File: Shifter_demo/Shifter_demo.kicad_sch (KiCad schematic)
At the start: 37 parts, among them IC1 BD450M2WFP3-CE2, IC2 LMR50410Y3FQDBVRQ1, J1 GT-USB-7010AN, SW1 TL3302BF180QG, SW2 TL3302BF180QG, U1 RP2040, U3 W25Q128JVSIQ, X1 XTAL12MHZ

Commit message: Add files via upload
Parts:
- added D1: RED LED, LED_SMD:LED_0805_2012Metric_Pad1.15x1.40mm_HandSolder, symbol Device:LED
- added D2: GREEN LED, LED_SMD:LED_0805_2012Metric_Pad1.15x1.40mm_HandSolder, symbol Device:LED
- added D3: BLUE LED, LED_SMD:LED_0805_2012Metric_Pad1.15x1.40mm_HandSolder, symbol Device:LED
- added J2, J3: B03B-XASK-1_LF__SN_, Connector_JST:JST_XA_B03B-XASK-1_1x03_P2.50mm_Vertical, symbol B03B-XASK-1_LF__SN_:B03B-XASK-1_LF__SN_
- added R10: 270R, Resistor_SMD:R_0805_2012Metric_Pad1.20x1.40mm_HandSolder, symbol Device:R
- added R11: 220R, Resistor_SMD:R_0805_2012Metric_Pad1.20x1.40mm_HandSolder, symbol Device:R
- added R13: 100R, Resistor_SMD:R_0805_2012Metric_Pad1.20x1.40mm_HandSolder, symbol Device:R
- added S1, S2: KMR731NG_LFS, KMR731NG LFS:KMR731NGLFS, symbol KMR731NG_LFS:KMR731NG_LFS
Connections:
- net +3V3: now also R10.1
- net GND: now also D1.1 (K), D2.1 (K), D3.1 (K), J2.1, J3.1, S1.1 (NO_1), S1.2 (NO_2), S1.3 (COM_1), S2.1 (NO_1), S2.2 (NO_2), S2.3 (COM_1)
- net Test_UP_Button: now reaches U1.3 (GPIO1)
- net Test_UP_Button: now also S1.4 (COM_2)
- net Test_DOWN_Button: now reaches U1.4 (GPIO2)
- net Test_DOWN_Button: now also S2.4 (COM_2)
- net UP_Button: now reaches U1.5 (GPIO3)
- net DOWN_Button: now reaches U1.6 (GPIO4)
- net DOWN_LED: now reaches U1.8 (GPIO6)
- net DOWN_LED: now also R13.1
- net UP_LED: now reaches U1.9 (GPIO7)
- net UP_LED: now also R11.1
- new net: D1.2 (A), R10.2
- new net: D3.2 (A), R13.2
- new net: D2.2 (A), R11.2
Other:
- note added: "Buttons"
- note added: "ECU wires can be 5-14 V + nasty spikes, so cant connect directly. aka we need to use interface circuitry For analog sensors: high-value voltage divider + RC filter so the RP2040s ADC never sees over 3.3 V and doesn't load the sensor. For buses like CAN/LIN, we need proper transceiver ICs."
- note added: "I went with: POWER: RED(Constant) UP: GREEN(One Blink) DOWN: BLUE(One Blink)"
- note added: "Idk what u want to conect here, but there u are:"
- note added: "JST XAs"
- note added: "LEDs"
- note added: "Original"
- note added: "The buttons are active low"
- moved on the sheet: C1, C10, C11, C12, C13, C14, C15, C16, C17, C18, C2, C3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

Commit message: Update Schematic
Adds ESP32, CAN and basically everything...
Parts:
- removed C1, C9: 1u, C0603, symbol Reference_import-altium-import:root_3_CL10A105KB8NNNC_
- removed C10, C11, C14: 100n, C0603, symbol Reference_import-altium-import:root_1_CC0603KRX7R9BB104_
- removed C12, C13: 27P, C0603, symbol Reference_import-altium-import:root_0_CL10C270JB8NNNC_
- removed C2, C3, C4, C5, C6, C7, C8: 100n, C0603, symbol Reference_import-altium-import:root_3_CC0603KRX7R9BB104_
- removed IC1: BD450M2WFP3-CE2, SOT230P700X170-4N, symbol BD450M2WFP3-CE2:BD450M2WFP3-CE2
- removed J1: GT-USB-7010AN, USB-SMD_GT-USB-7010AN, symbol Reference_import-altium-import:root_0_GT-USB-7010AN_
- removed J2, J3: B03B-XASK-1_LF__SN_, Connector_JST:JST_XA_B03B-XASK-1_1x03_P2.50mm_Vertical, symbol B03B-XASK-1_LF__SN_:B03B-XASK-1_LF__SN_
- removed R1, R2: 27, R0603, symbol Reference_import-altium-import:root_0_0603WAF270JT5E_
- removed R12: 10k, R0603, symbol Reference_import-altium-import:root_1_0603WAF1002T5E_
- removed R3, R5: 1k, R0603, symbol Reference_import-altium-import:root_0_0603WAF1001T5E_
- removed R4: 10k - DNF, R0603, symbol Reference_import-altium-import:root_1_10k - DNF_
- removed S1, S2: KMR731NG_LFS, KMR731NG LFS:KMR731NGLFS, symbol KMR731NG_LFS:KMR731NG_LFS
- removed SW1: TL3302BF180QG, SW-SMD_L6.0-W3.5-LS10.2, symbol Reference_import-altium-import:root_0_TL3302BF180QG_
- removed SW2: TL3302BF180QG, SW-SMD_L6.0-W3.5-LS10.2, symbol Reference_import-altium-import:root_1_TL3302BF180QG_
- removed U1: RP2040, symbol Reference_import-altium-import:root_0_RP2040_
- removed U3: W25Q128JVSIQ, SOIC-8_L5.3-W5.3-P1.27-LS8.0-BL, symbol Reference_import-altium-import:root_0_W25Q128JVSSIQ_
- removed X1: XTAL12MHZ, CRYSTAL-SMD_4P-L2.5-W2.0-BL_XTAL12MHZ, symbol Reference_import-altium-import:root_0_XTAL12MHz_
- added C1, C5: 1u, symbol Device:C
- added C2: 22u, symbol Device:C
- added C3, C4, C6, C7, C8: 0.1u, symbol Device:C
- added D4: RED LED, LED_SMD:LED_0805_2012Metric_Pad1.15x1.40mm_HandSolder, symbol Device:LED
- added J1: RST, symbol Connector_Generic:Conn_01x02
- added J2: BSEL, symbol Connector_Generic:Conn_01x02
- added J3: S06B-XASK-1, symbol Connector_Generic:Conn_01x06
- added J4: SO4B-XASK-1, symbol Connector_Generic:Conn_01x04
- added J5, J6: S03B-XASK-1, symbol Connector_Generic:Conn_01x03
- added Q1: BSS205N, Custom_MSM:MOSFET_Single_SOT-23, symbol Custom_MSM:MOSFET_N-CH
- added R1, R2: 27, symbol Device:R
- added R3: 10k, symbol Device:R
- added R4: 270R, Resistor_SMD:R_0805_2012Metric_Pad1.20x1.40mm_HandSolder, symbol Device:R
- added U1: ESP32-S3-WROOM-1U-N4R2, ESP32-S3-WROOM-1U-N4R2:XCVR_ESP32-S3-WROOM-1U-N4R2, symbol ESP32-S3-WROOM-1U-N4R2:ESP32-S3-WROOM-1U-N4R2
- added U3: MAX3390EEUD_T, MAX3390EEUD_T:SOP65P640X110-14N, symbol MAX3390EEUD_T:MAX3390EEUD_T
- added U4: ISO1042BQDWVQ1, DWV0008A-IPC_A, symbol 2025-11-15_02-18-59:ISO1042BQDWVQ1
- added USB1: GT-USB-7010AN, USB-SMD_GT-USB-7010AN, symbol Reference_import-altium-import:root_0_GT-USB-7010AN_
- renumbered IC2 to U2
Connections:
- net +3V3: now also C2.2, C3.2, C6.1, C8.2, R3.1, U1.2 (3V3), U3.1 (VL), U3.8 (~{THREE}-STATE), U4.1 (VCC1)
- net +5V: now also C4.1, C5.1, C7.2, J3.6 (Pin_6), J5.3 (Pin_3), U3.14 (VCC), U4.8 (VCC2), USB1.A4B9 (VBUS), USB1.B4A9 (VBUS)
- net DOWN_LED: now also U1.7 (IO7)
- net GND: now also C1.1, C2.1, C3.1, C4.2, C5.2, C6.2, C7.1, C8.1, D4.1 (K), J1.1 (Pin_1), J2.1 (Pin_1), J3.1 (Pin_1), J5.1 (Pin_1), J6.1 (Pin_1), Q1.2 (S), U1.1 (GND), U1.40 (GND__1), U1.41_1 (GND__2), U1.41_2 (GND__3), U1.41_3 (GND__4), U1.41_4 (GND__5), U1.41_5 (GND__6), U1.41_6 (GND__7), U1.41_7 (GND__8), U1.41_8 (GND__9), U1.41_9 (GND__10), U3.7 (GND), U4.4 (GND1), U4.5 (GND2), USB1.13 (GND), USB1.14 (GND), USB1.15 (GND), USB1.16 (GND), USB1.A1B12 (GND), USB1.B1A12 (GND)
- net SCLK: now also U1.20 (IO12), U3.4 (I_VL3)
- net UP_LED: now also U1.6 (IO6)
- net USBD+: now also R2.2, USB1.A6 (DP1), USB1.B6 (DP2)
- net USBD-: now also R1.2, USB1.A7 (DN1), USB1.B7 (DN2)
- net at R8.2: now also USB1.A5 (CC1)
- net at R7.2: now also USB1.B5 (CC2)
- new net: R1.1, U1.13 (IO19)
- new net: D4.2 (A), R4.2
- new net: R2.1, U1.14 (IO20)
- new net: J2.2 (Pin_2), U1.27 (IO0)
- new net CAND: U1.39 (IO1), U4.2 (TXD)
- new net CANH: J6.3 (Pin_3), U4.7 (CANH)
- new net CANL: J6.2 (Pin_2), U4.6 (CANL)
- new net CANR: U1.38 (IO2), U4.3 (RXD)
- new net CS: U1.18 (IO10), U3.5 (I_VL4)
- new net ECU: J4.4 (Pin_4), Q1.3 (D)
- new net E_CS: J3.5 (Pin_5), U3.10 (O_VCC4)
- new net E_MISO: J3.3 (Pin_3), U3.13 (I_VCC1)
- new net E_MOSI: J3.4 (Pin_4), U3.12 (O_VCC2)
- new net E_SCLK: J3.2 (Pin_2), U3.11 (O_VCC3)
- new net FLATSHIFT: Q1.1 (G), U1.5 (IO5)
- new net MISO: U1.21 (IO13), U3.2 (O_VL1)
- new net MOSI: U1.19 (IO11), U3.3 (I_VL2)
- new net Main_Reset: C1.2, J1.2 (Pin_2), R3.2, U1.3 (EN)
- new net NEUTRAL: J4.1 (Pin_1)
- new net NEUTRAL_LED: R4.1, U1.12 (IO8)
- new net PWM: J5.2 (Pin_2)
- new net RX: U1.36 (RXD0)
- new net SHIFT_DOWN: J4.2 (Pin_2)
- new net SHIFT_UP: J4.3 (Pin_3)
- new net TX: U1.37 (TXD0)
- no-connect marks 32 -> 23
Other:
- note added: "CAN"
- note added: "CAN (Rest of Car)"
- note added: "ECU"
- note added: "ESC"
- note added: "Encoder"
- note added: "Encoder Interface"
- note added: "Microcontroller"
- note added: "REG"
- note added: "Rest of Car"
- note added: "USB"
- note removed: "Buttons"
- note removed: "C1 must be near Pin 44"
- note removed: "C9 must be near Pin 45"
- note removed: "ECU wires can be 5-14 V + nasty spikes, so cant connect directly. aka we need to use interface circuitry For analog sensors: high-value voltage divider + RC filter so the RP2040s ADC never sees over 3.3 V and doesn't load the sensor. For buses like CAN/LIN, we need proper transceiver ICs."
- note removed: "Idk what u want to conect here, but there u are:"
- note removed: "Linear Batt to 5V reg"
- note removed: "On-PCB shifter buttons (For testing) ECU signal line (research required) Status Lights Connectors (JST XA)"
- note removed: "Original"
- note removed: "R1 and R2 must be near RP2040"
- note removed: "RP2040 Microcontroller"
- note removed: "SPI Flash"
- note removed: "Switching 5V to 3V3 reg"
- note removed: "The buttons are active low"
- note removed: "Todo:"
- note removed: "Try to match crystal track length"
- note removed: "USB BOOT (Pull Low)"
- moved on the sheet: C15, C16, C17, C18, D1, D2, D3, L1, R10, R11, R13, R6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

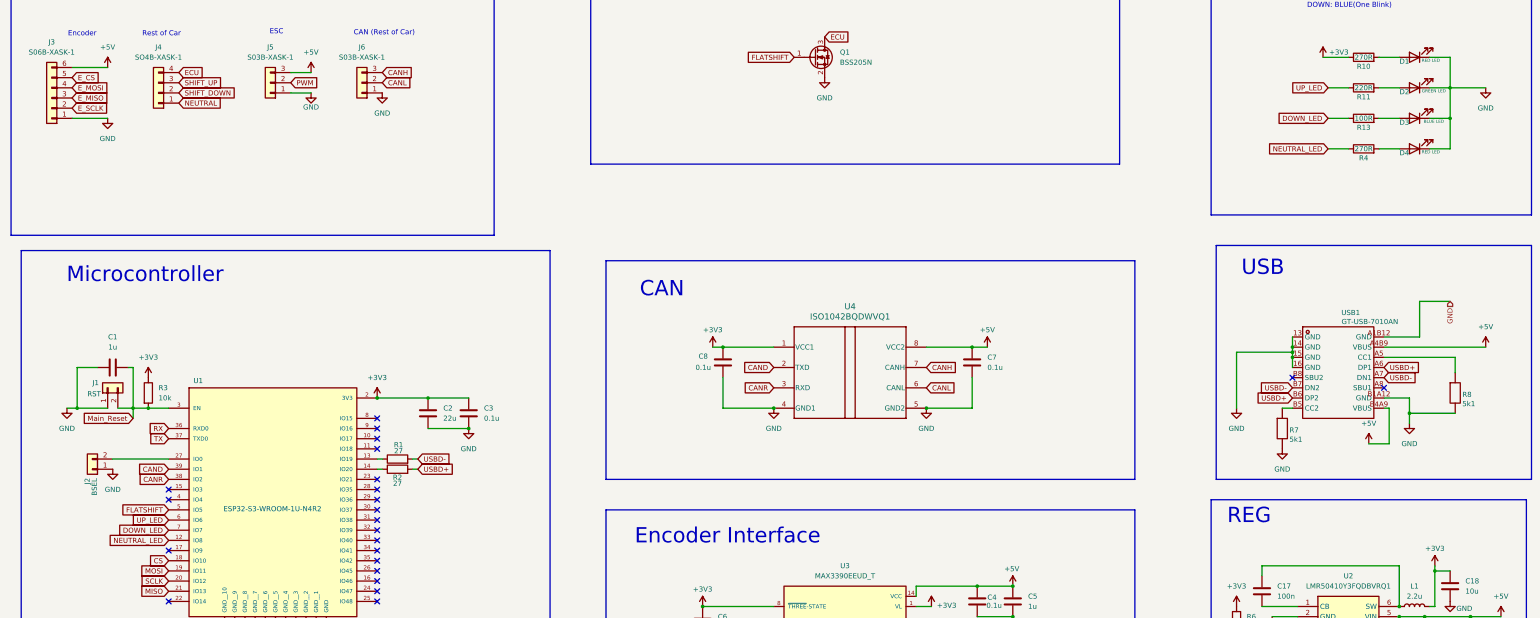
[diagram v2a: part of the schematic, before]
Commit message: route it all and make minor schem mods
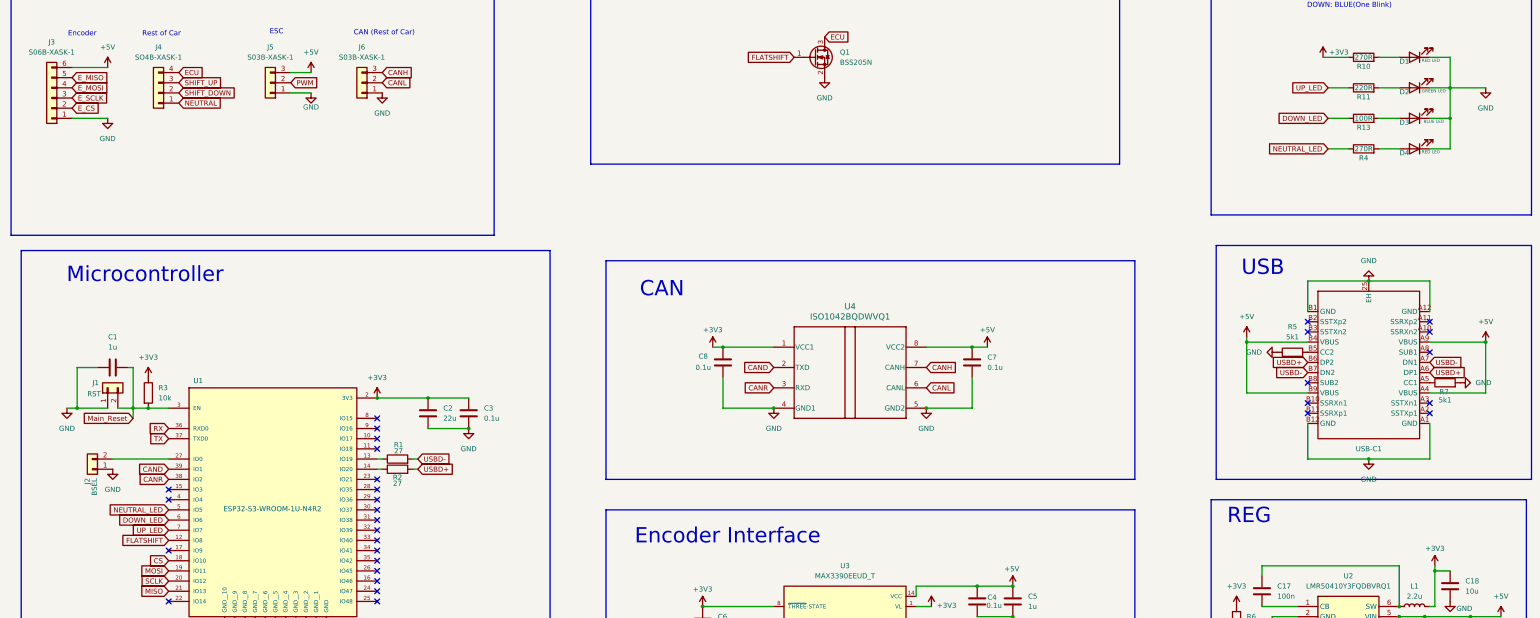
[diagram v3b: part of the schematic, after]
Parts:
- removed R7, R8: 5k1, R0603, symbol Reference_import-altium-import:root_1_0603WAF5101T5E_
- removed USB1: GT-USB-7010AN, USB-SMD_GT-USB-7010AN, symbol Reference_import-altium-import:root_0_GT-USB-7010AN_
- added R5, R7: 5k1, Resistor_SMD:R_0805_2012Metric_Pad1.20x1.40mm_HandSolder, symbol Device:R
- added USB-C1: ~, CustomFootprints:USB-C, symbol USB-C:USB_1
- C1, C15, C16, C17, C18, C2, C3, C4, C5, C6, C7, C8: footprint (none) -> Capacitor_SMD:C_0805_2012Metric_Pad1.18x1.45mm_HandSolder
- J1, J2: footprint (none) -> Connector_PinHeader_2.54mm:PinHeader_1x02_P2.54mm_Vertical
- J3: footprint (none) -> Connector_JST:JST_XA_S06B-XASK-1_1x06_P2.50mm_Horizontal
- J4: footprint (none) -> Connector_JST:JST_XA_S04B-XASK-1_1x04_P2.50mm_Horizontal
- J5, J6: footprint (none) -> Connector_JST:JST_XA_S03B-XASK-1_1x03_P2.50mm_Horizontal
- L1: footprint (none) -> Inductor_SMD:L_0805_2012Metric_Pad1.15x1.40mm_HandSolder
- R1, R2, R3, R6, R9: footprint (none) -> Resistor_SMD:R_0805_2012Metric_Pad1.20x1.40mm_HandSolder
- U1: footprint ESP32-S3-WROOM-1U-N4R2:XCVR_ESP32-S3-WROOM-1U-N4R2 -> CustomFootprints:XCVR_ESP32-S3-WROOM-1U-N4R2
- U2: footprint SOT95P280X145-6N -> CustomFootprints:SOT95P280X145-6N
- U3: footprint MAX3390EEUD_T:SOP65P640X110-14N -> CustomFootprints:SOP65P640X110-14N
- U4: footprint DWV0008A-IPC_A -> CustomFootprints:DWV0008A-MFG
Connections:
- net +5V: now also USB-C1.A4 (VBUS), USB-C1.A9 (VBUS), USB-C1.B4 (VBUS), USB-C1.B9 (VBUS)
- net DOWN_LED: now also U1.6 (IO6); no longer U1.7 (IO7)
- net E_CS: now also J3.2 (Pin_2); no longer J3.5 (Pin_5)
- net E_MISO: now also J3.5 (Pin_5); no longer J3.3 (Pin_3)
- net E_SCLK: now also J3.3 (Pin_3); no longer J3.2 (Pin_2)
- net FLATSHIFT: now also U1.12 (IO8); no longer U1.5 (IO5)
- net GND: now also R5.1, R7.2, USB-C1.25 (EH), USB-C1.A1 (GND), USB-C1.A12 (GND), USB-C1.B1 (GND), USB-C1.B12 (GND)
- net NEUTRAL_LED: now also U1.5 (IO5); no longer U1.12 (IO8)
- net UP_LED: now also U1.7 (IO7); no longer U1.6 (IO6)
- net USBD+: now also USB-C1.A6 (DP1), USB-C1.B6 (DP2)
- net USBD-: now also USB-C1.A7 (DN1), USB-C1.B7 (DN2)
- new net: R7.1, USB-C1.A5 (CC1)
- new net: R5.2, USB-C1.B5 (CC2)
- no-connect marks 23 -> 31

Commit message: Add SCS checks to Schematic and PCB
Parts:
- removed J3: S06B-XASK-1, Connector_JST:JST_XA_S06B-XASK-1_1x06_P2.50mm_Horizontal, symbol Connector_Generic:Conn_01x06
- removed J6: S03B-XASK-1, Connector_JST:JST_XA_S03B-XASK-1_1x03_P2.50mm_Horizontal, symbol Connector_Generic:Conn_01x03
- added J3, J7: S03B-XASK-1, Connector_JST:JST_XA_S03B-XASK-1_1x03_P2.50mm_Horizontal, symbol Connector_Generic:Conn_01x03
- added J6: SO4B-XASK-1, Connector_JST:JST_XA_S04B-XASK-1_1x04_P2.50mm_Horizontal, symbol Connector_Generic:Conn_01x04
- added R12, R14, R15, R16, R17, R18, R19, R20, R25, R27, R8: 10k, Resistor_SMD:R_0805_2012Metric_Pad1.20x1.40mm_HandSolder, symbol Device:R
- added R21, R22, R23: 180, Resistor_SMD:R_0805_2012Metric_Pad1.20x1.40mm_HandSolder, symbol Device:R
- added R24: 5k8, Resistor_SMD:R_0805_2012Metric_Pad1.20x1.40mm_HandSolder, symbol Device:R
- added R26: 12k, Resistor_SMD:R_0805_2012Metric_Pad1.20x1.40mm_HandSolder, symbol Device:R
- added TP1, TP10, TP11, TP12, TP2, TP3, TP4, TP5, TP6, TP7, TP8, TP9: TestPoint, TestPoint:TestPoint_Pad_D1.0mm, symbol Connector:TestPoint
- added U5, U6: LM339, CustomFootprints:LM339DR, symbol Comparator:LM339
- added U8: CD4081, CustomFootprints:D14, symbol 74xx:74LS09
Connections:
- net +3V3: now also J4.4 (Pin_4), R14.2, R15.1, R17.2, R18.2, R19.1, R20.1, U8.14 (VCC)
- net +5V: now also J3.3 (Pin_3), R24.1, R26.1, U5.3 (V+), U6.3 (V+)
- net CANH: now also J6.3 (Pin_3)
- net CANL: now also J6.2 (Pin_2)
- net ECU: now also J6.4 (Pin_4); no longer J4.4 (Pin_4)
- net E_CS: now also J7.2 (Pin_2)
- net E_MISO: now also J3.2 (Pin_2)
- net E_MOSI: now also J3.1 (Pin_1)
- net E_SCLK: now also J7.3 (Pin_3)
- net GND: now also J6.1 (Pin_1), J7.1 (Pin_1), R12.2, R16.2, R25.2, R27.2, R8.2, U5.12 (V-), U6.12 (V-), U8.7 (GND)
- net NEUTRAL: now also U1.26 (IO45), TP12.1, U8.8; no longer J4.1 (Pin_1)
- net SHIFT_DOWN: now also R21.1
- net SHIFT_UP: now also R23.1
- net UP: now reaches U1.24 (IO47)
- net UP: now also TP9.1, U8.3
- net DOWN: now reaches U1.25 (IO48)
- net DOWN: now also TP7.1, U8.6
- new net: R20.2, U6.1, U8.10
- new net: R16.1, R22.2, TP10.1, U6.4 (-), U6.7 (+)
- new net: R14.1, U5.13, U8.4
- new net: R15.2, U5.14, U8.5
- new net: R23.2, R8.1, TP4.1, U5.4 (-), U5.7 (+)
- new net: R18.1, U5.2, U8.1
- new net: R19.2, U5.1, U8.2
- new net: R12.1, R21.2, TP2.1, U5.10 (-), U5.9 (+)
- new net: R17.1, U6.2, U8.9
- new net 2.5V Ref: R26.2, R27.1, TP11.1, TP5.1, TP6.1, U5.6 (-), U5.8 (-), U6.6 (-)
- new net 3.5V Ref: R24.2, R25.1, TP1.1, TP3.1, TP8.1, U5.11 (+), U5.5 (+), U6.5 (+)
- new net SHIFT_NEUTRAL: J4.1 (Pin_1), R22.1
- no-connect marks 31 -> 28
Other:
- note added: "References, Power supplys"
- note added: "SCS checks"
- note removed: "I went with: POWER: RED(Constant) UP: GREEN(One Blink) DOWN: BLUE(One Blink)"
- moved on the sheet: C15, C16, C17, C18, C4, C5, C6, C7, C8, D1, D2, D3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
